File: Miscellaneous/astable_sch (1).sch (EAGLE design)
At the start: 6 parts, among them IC1 LM555N

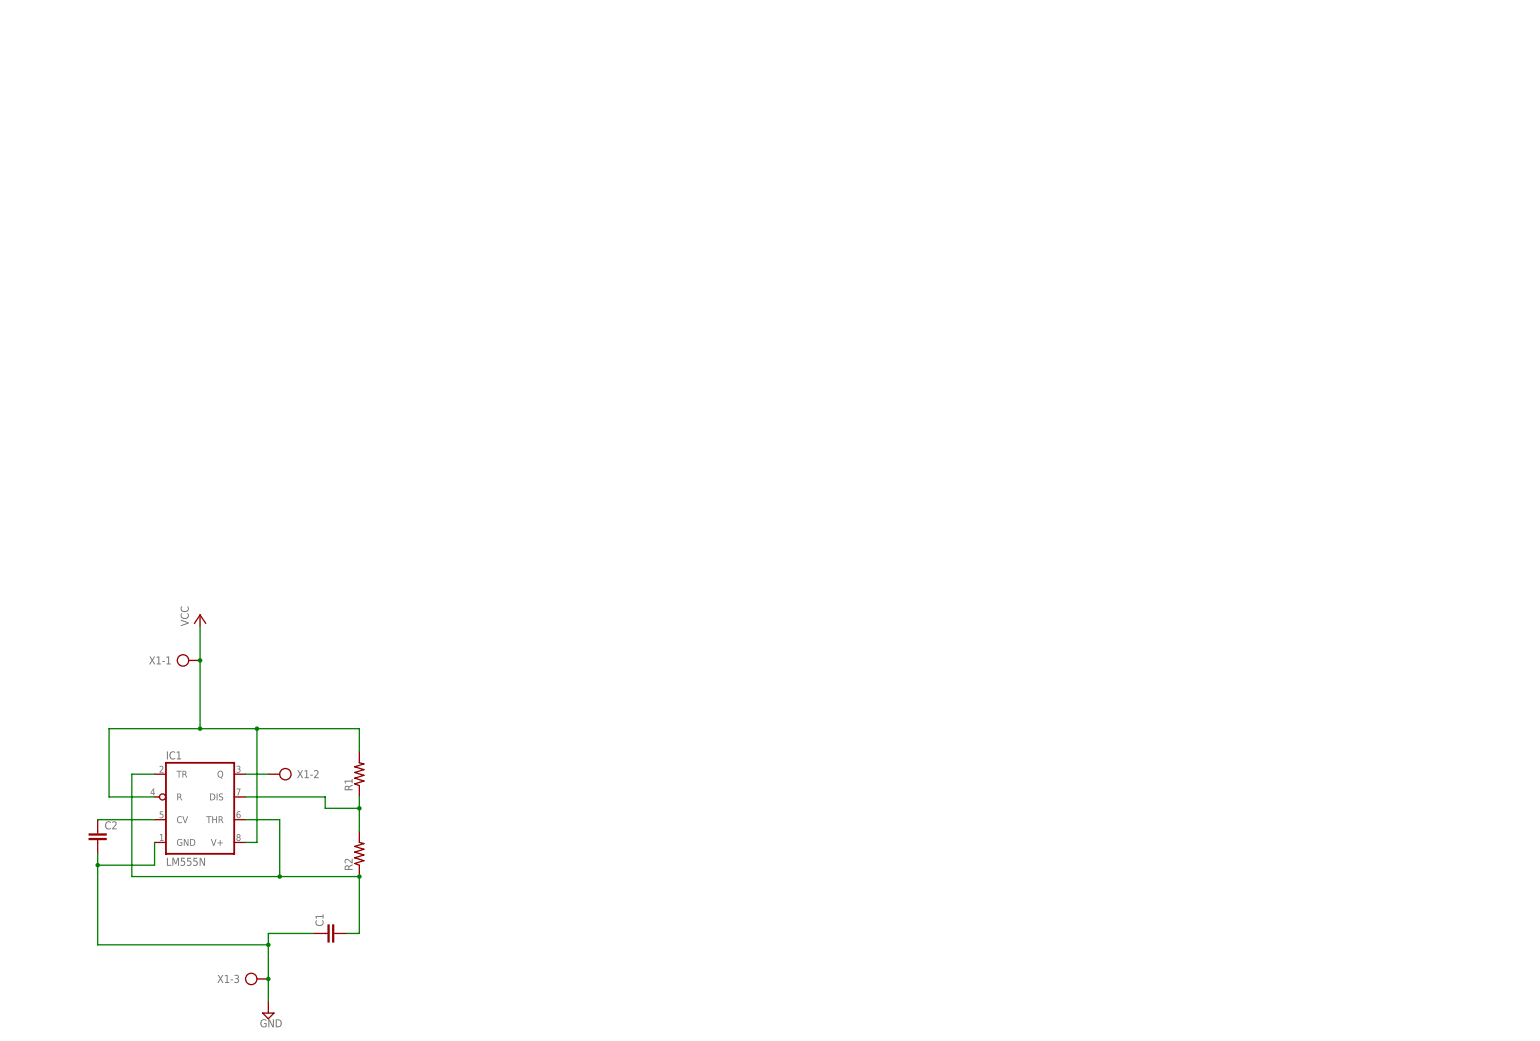
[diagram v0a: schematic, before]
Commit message: Fixed the PCB design
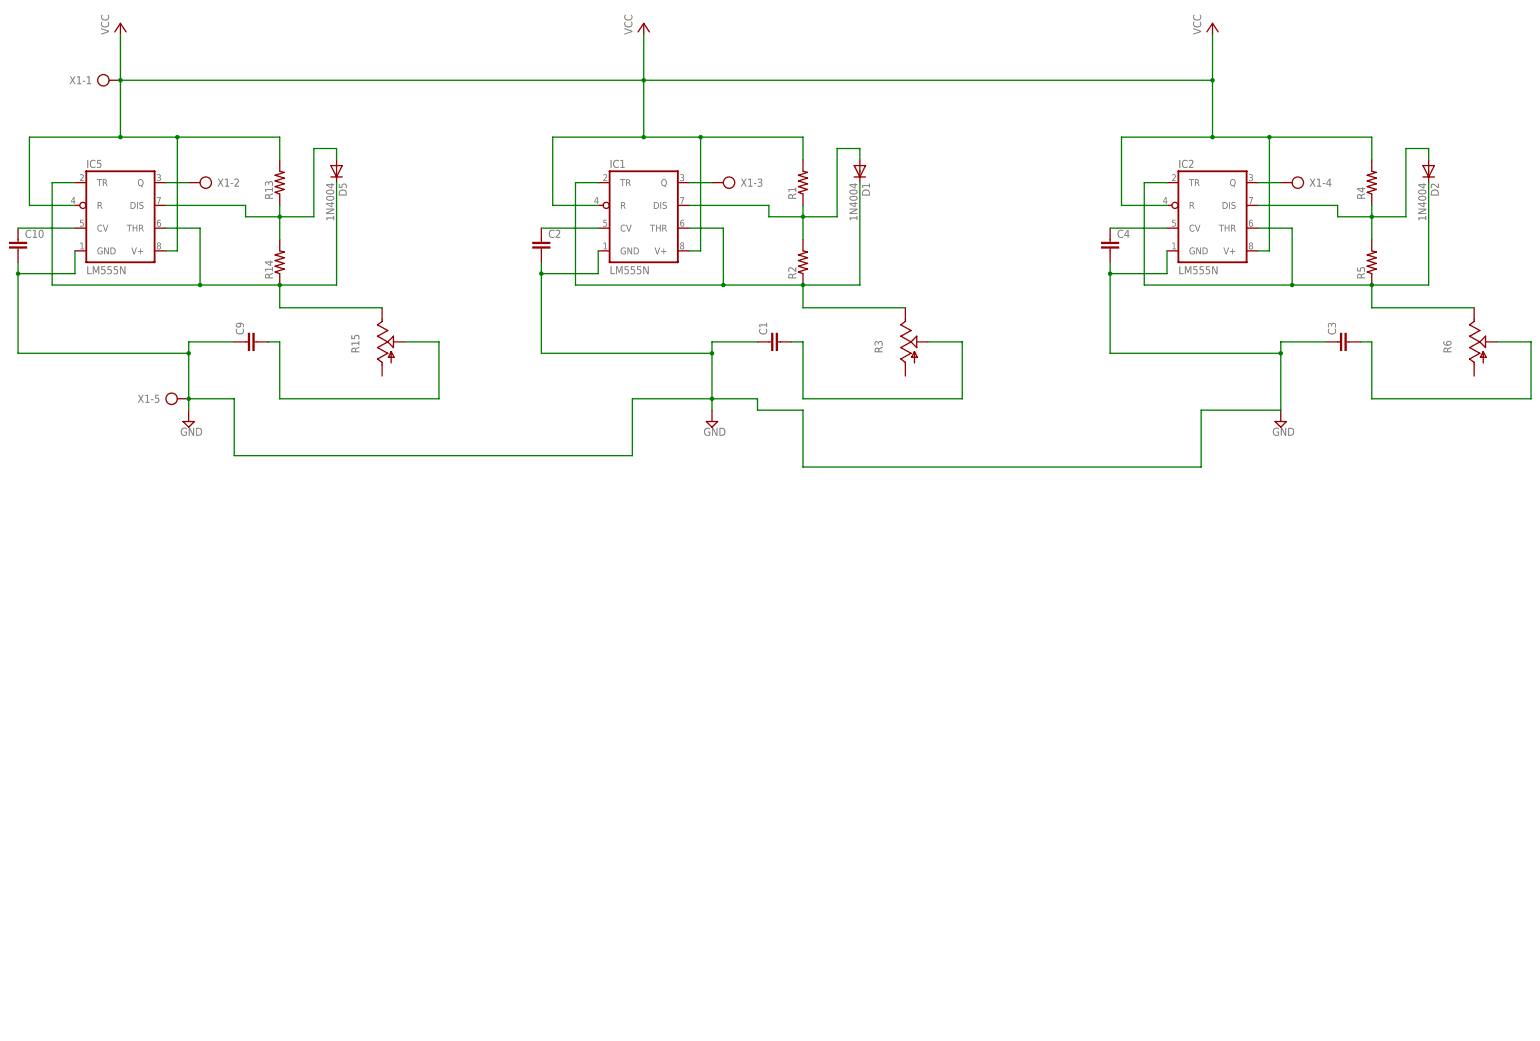
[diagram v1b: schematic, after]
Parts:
- added C10, C3, C4, C9: (no value), rcl:C-EU025-024X044
- added D1, D2, D5: 1N4004, diode:1N4004
- added IC2, IC5: LM555N, linear:LM555N
- added R13, R14, R4, R5: (no value), rcl:R-US_0204/7
- added R15, R3, R6: (no value), pot:TRIM_US-B25V
- X1: device con-ptr500:AK300/3 -> con-ptr500:AK300/5
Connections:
- new net N$1: D1.A, IC1.DIS, R1.1, R2.2
- new net N$10: C3.2, R6.S
- new net N$21: D5.A, IC5.DIS, R13.1, R14.2
- new net N$22: D5.C, IC5.THR, IC5.TR, R14.1, R15.E
- new net N$23: C10.1, IC5.CV
- new net N$24: IC5.Q, X1-2.KL
- new net N$25: C9.2, R15.S
- new net N$5: C1.2, R3.S
- new net N$6: D2.A, IC2.DIS, R4.1, R5.2
- new net N$7: D2.C, IC2.THR, IC2.TR, R5.1, R6.E
- new net N$8: C4.1, IC2.CV
- net GND: now also C10.2, C3.1, C4.2, C9.1, IC2.GND, IC5.GND, X1-5.KL; no longer X1-3.KL
- net N$2: now also D1.C, IC1.THR, IC1.TR, R2.1, R3.E; no longer IC1.DIS, R1.1, R2.2
- net N$4: now also IC1.Q, X1-3.KL; no longer C1.2, IC1.THR, IC1.TR, R2.1
- net N$9: now also IC2.Q, X1-4.KL; no longer IC1.Q, X1-2.KL
- net VCC: now also IC2.R, IC2.V+, IC5.R, IC5.V+, R13.2, R4.2
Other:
- moved on the sheet: C1, C2, IC1, R1, R2, X1-1, X1-2, X1-3

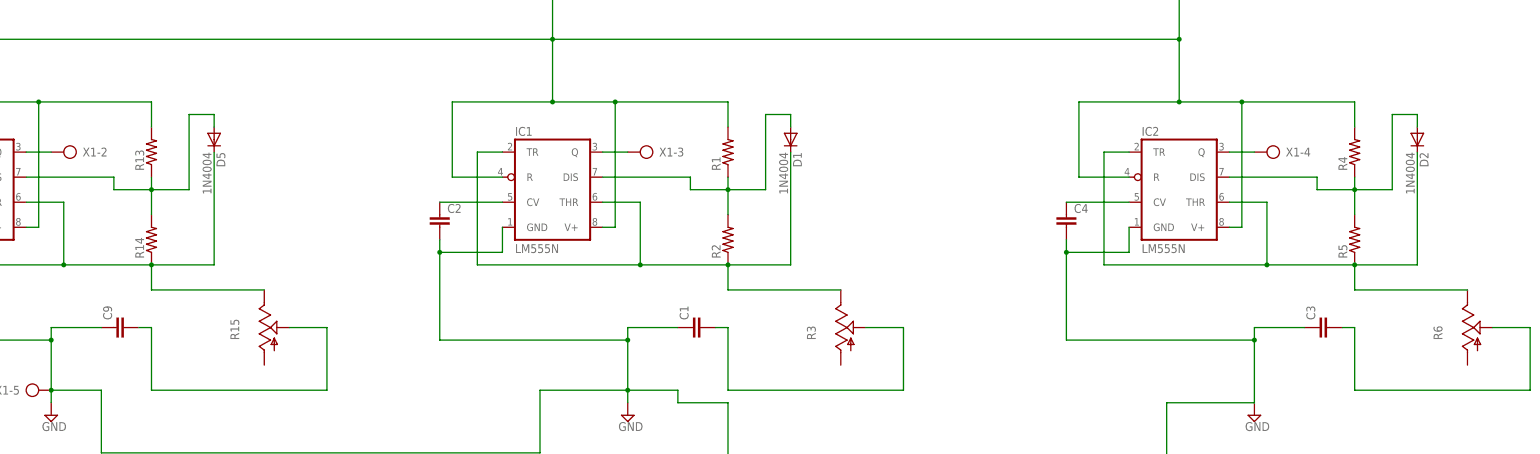
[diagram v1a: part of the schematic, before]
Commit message: Updated the PCB Design
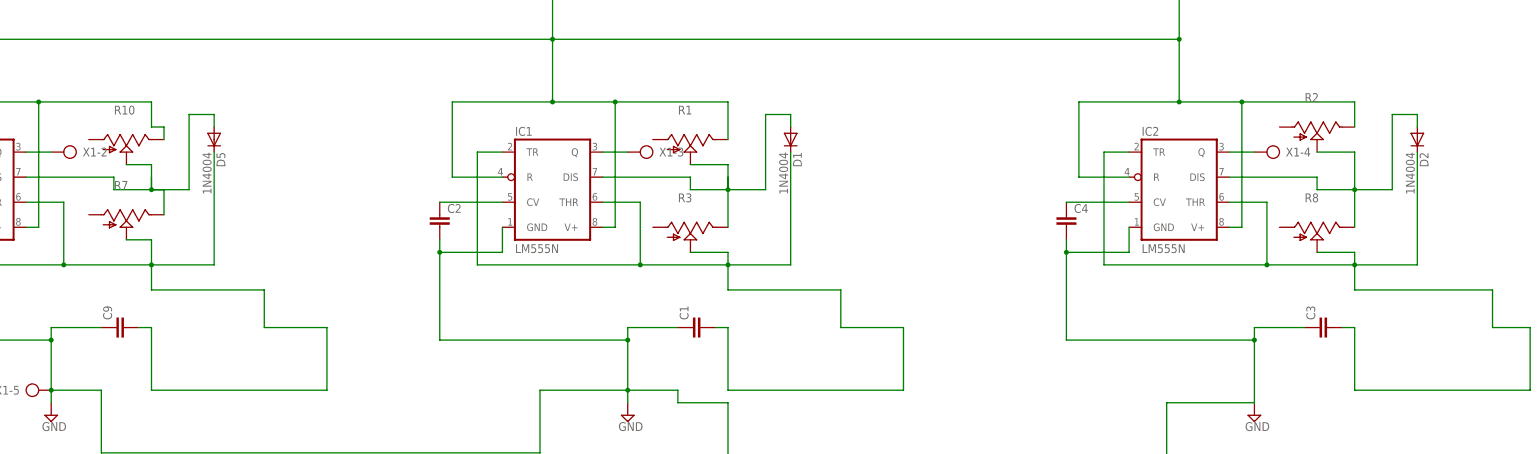
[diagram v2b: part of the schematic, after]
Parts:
- removed R13, R14, R4, R5: (no value), rcl:R-US_0204/7
- removed R15, R6: (no value), pot:TRIM_US-B25V
- added R10, R7, R8: (no value), pot:TRIM_US-B25V
- R1, R2: device rcl:R-US_0204/7 -> pot:TRIM_US-B25V
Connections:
- removed net N$10: C3.2, R6.S
- removed net N$25: C9.2, R15.S
- removed net N$5: C1.2, R3.S
- net N$1: now also R1.S, R3.E; no longer R1.1, R2.2
- net N$2: now also C1.2, R3.S; no longer R2.1, R3.E
- net N$21: now also R10.S, R7.E; no longer R13.1, R14.2
- net N$22: now also C9.2, R7.S; no longer R14.1, R15.E
- net N$6: now also R2.S, R8.E; no longer R4.1, R5.2
- net N$7: now also C3.2, R8.S; no longer R5.1, R6.E
- net VCC: now also R1.E, R10.E, R2.E; no longer R1.2, R13.2, R4.2
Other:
- moved on the sheet: R3
